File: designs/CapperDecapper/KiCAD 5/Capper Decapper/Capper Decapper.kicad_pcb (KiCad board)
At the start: 2 copper layers, 94 x 61.6 mm, 50 parts, among them J1 Screw_Terminal_01x02, J2 Conn_01x03_Female, J3 Analog_Zero, J4 Pi_Signals, J5 Motor_Power, Q1 Q_NMOS_GDS, U1 L2293, U10 INA214, U11 L2293, U12 INA214, U13 INA214, U14 LM338-ADJ, U2 INA214, U3 INA214, U4 L2293, U5 INA214, U6 INA214, U7 ADP172, U8 L2293, U9 INA214

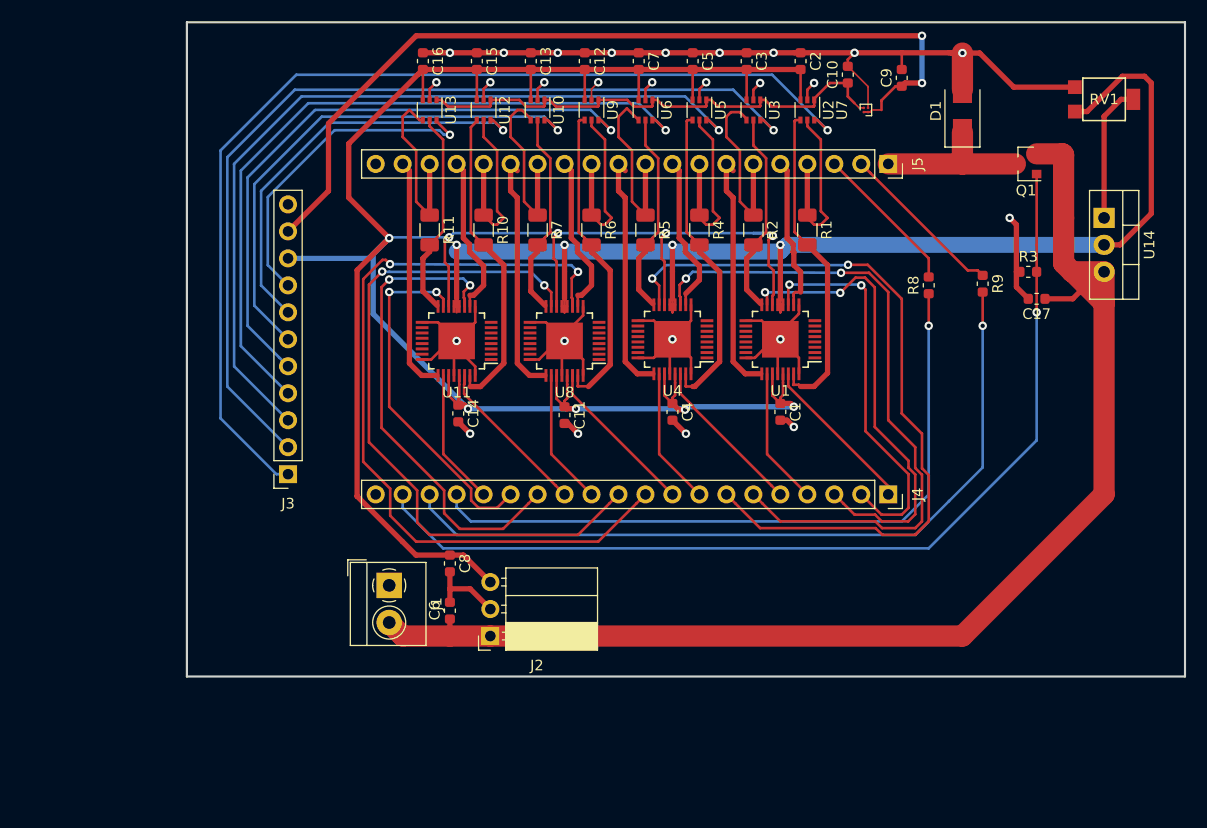
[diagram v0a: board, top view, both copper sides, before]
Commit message: PWM capper decapper board
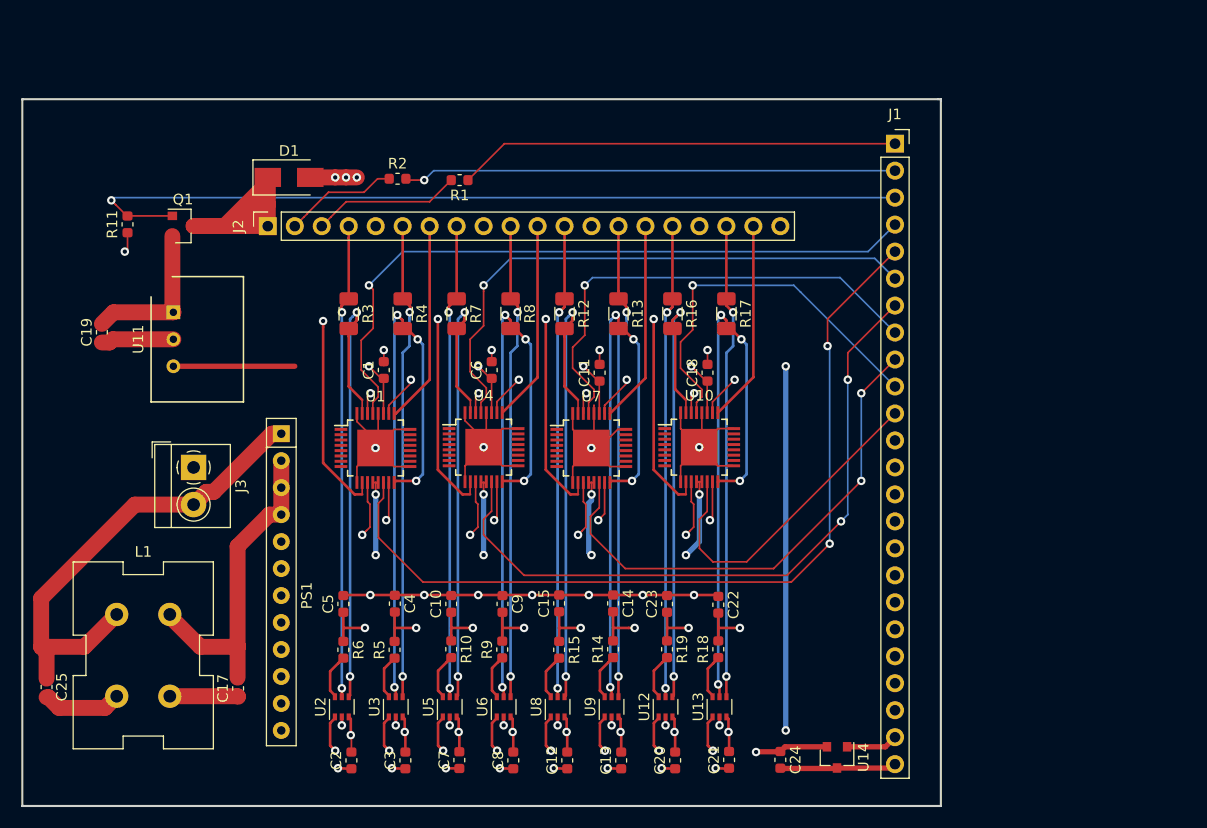
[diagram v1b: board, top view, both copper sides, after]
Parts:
- removed C16: C, Capacitor_SMD:C_0603_1608Metric
- removed J4: Pi_Signals, Connector_PinSocket_2.54mm:PinSocket_1x20_P2.54mm_Vertical
- removed J5: Motor_Power, Connector_PinSocket_2.54mm:PinSocket_1x20_P2.54mm_Vertical
- removed RV1: R_POT, CustomFootprints:R_TRIM_4mm_Gull
- added C18: 0.01uF, Capacitor_SMD:C_0603_1608Metric, F.Cu at (148.1, 60.3)
- added C19: 0.1uF, Capacitor_SMD:C_0603_1608Metric, F.Cu at (91.1, 56.5)
- added C20: 0.1uF, Capacitor_SMD:C_0603_1608Metric, F.Cu at (145.0, 96.8)
- added C21: 0.1uF, Capacitor_SMD:C_0603_1608Metric, F.Cu at (150.1, 96.7)
- added C22: 22nF, Capacitor_SMD:C_0603_1608Metric, F.Cu at (149.1, 82.1)
- added C23: 22nF, Capacitor_SMD:C_0603_1608Metric, F.Cu at (144.3, 82.1)
- added C24: 0.01uF, Capacitor_SMD:C_0603_1608Metric, F.Cu at (154.9, 96.7)
- added C25: 33uF, Capacitor_SMD:C_0603_1608Metric, F.Cu at (85.9, 89.9)
- added L1: L_Coupled, Inductor_THT:L_CommonMode_Wuerth_WE-CMB-S, F.Cu at (92.5, 83.1)
- added PS1: R-7XX, Resistor_THT:R_Array_SIP12, F.Cu at (108.0, 66.0)
- added R12: 0.05R, Resistor_SMD:R_1206_3216Metric, F.Cu at (134.6, 54.7)
- added R13: 0.05R, Resistor_SMD:R_1206_3216Metric, F.Cu at (139.7, 54.7)
- added R14: 20k, Resistor_SMD:R_0603_1608Metric, F.Cu at (139.2, 86.3)
- added R15: 20k, Resistor_SMD:R_0603_1608Metric, F.Cu at (134.1, 86.4)
- added R16: 0.05R, Resistor_SMD:R_1206_3216Metric, F.Cu at (144.8, 54.7)
- added R17: 0.05R, Resistor_SMD:R_1206_3216Metric, F.Cu at (149.9, 54.7)
- added R18: 20k, Resistor_SMD:R_0603_1608Metric, F.Cu at (149.1, 86.3)
- added R19: 20K, Resistor_SMD:R_0603_1608Metric, F.Cu at (144.3, 86.3)
- C1, C11, C7: value C -> 0.01uF
- C10, C14, C15, C4, C5, C9: value C -> 22nF
- C12, C13, C2, C3, C6, C8: value C -> 0.1uF
- C17: value C -> 33uF
- D1: value D_Schottky_Small_ALT -> Schottky
- J1: value Screw_Terminal_01x02 -> Pi Control Signals; footprint TerminalBlock_4Ucon:TerminalBlock_4Ucon_1x02_P3.50mm_Horizontal -> Connector_PinSocket_2.54mm:PinSocket_1x24_P2.54mm_Vertical
- J2: value Conn_01x03_Female -> Motor_Power; footprint Connector_PinSocket_2.54mm:PinSocket_1x03_P2.54mm_Horizontal -> Connector_PinSocket_2.54mm:PinSocket_1x20_P2.54mm_Vertical
- J3: value Analog_Zero -> Screw_Term; footprint Connector_PinSocket_2.54mm:PinSocket_1x11_P2.54mm_Vertical -> TerminalBlock_4Ucon:TerminalBlock_4Ucon_1x02_P3.50mm_Horizontal
- R1, R2: value R_US -> 330R; footprint Resistor_SMD:R_1206_3216Metric -> Resistor_SMD:R_0603_1608Metric
- R10, R5, R6: value R_US -> 20k; footprint Resistor_SMD:R_1206_3216Metric -> Resistor_SMD:R_0603_1608Metric
- R11: value R_US -> 5k; footprint Resistor_SMD:R_1206_3216Metric -> Resistor_SMD:R_0603_1608Metric
- R3, R8: value R_US -> 0.05R; footprint Resistor_SMD:R_0603_1608Metric -> Resistor_SMD:R_1206_3216Metric
- R4, R7: value R_US -> 0.05R
- R9: value R_US -> 20k
- U10: value INA214 -> L2293; footprint Package_TO_SOT_SMD:SOT-363_SC-70-6 -> Package_QFP:LQFP-32-1EP_5x5mm_P0.5mm_EP3.45x3.45mm
- U11: value L2293 -> V7805-1500R; footprint Package_QFP:LQFP-32-1EP_5x5mm_P0.5mm_EP3.45x3.45mm -> Package_SIP:SIP3_11.6x8.5mm
- U14: value LM338-ADJ -> MAX6018BEUR16; footprint Package_TO_SOT_THT:TO-220-3_Vertical -> Package_TO_SOT_SMD:SOT-23
- U7: value ADP172 -> L2293; footprint Package_BGA:WLP-4_0.86x0.86mm_P0.4mm -> Package_QFP:LQFP-32-1EP_5x5mm_P0.5mm_EP3.45x3.45mm
- U8: value L2293 -> INA214; footprint Package_QFP:LQFP-32-1EP_5x5mm_P0.5mm_EP3.45x3.45mm -> Package_TO_SOT_SMD:SOT-363_SC-70-6
- moved C17 83.7 mm to (103.9, 90.0), turned to 90 degrees
- moved Q1 79.6 mm to (98.7, 46.5), turned to 0 degrees
- moved C2 78.2 mm to (114.6, 96.8), turned to 90 degrees
- moved C3 73.3 mm to (119.6, 96.8), turned to 90 degrees
- moved U2 71.3 mm to (113.7, 91.8), turned to 90 degrees
- moved C7 67.9 mm to (124.7, 96.8), turned to 90 degrees
- moved C13 66.4 mm to (140.0, 96.8), turned to 90 degrees
- moved C12 65.9 mm to (134.9, 96.8), turned to 90 degrees
- moved U3 65.5 mm to (118.7, 91.8), turned to 90 degrees
- moved R3 64.1 mm to (114.3, 54.7), turned to 270 degrees
- moved D1 63.7 mm to (108.7, 41.9), turned to 0 degrees
- moved J1 63.2 mm to (165.7, 38.7), turned to 0 degrees
- moved U13 62.5 mm to (149.2, 91.8), turned to 90 degrees
- moved C10 62.3 mm to (124.0, 82.1)
- moved C9 62.2 mm to (128.8, 82.1), turned to 270 degrees
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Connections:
- C10 pad 1: /V_mon -> /ADC3
- C14 pad 1: /5V -> GND
- C14 pad 2: GND -> /ADC6
- C15 pad 1: GND -> /ADC5
- C15 pad 2: /5V -> GND
- C17 pad 1: +36V -> GND
- C17 pad 2: GND -> Net-(C17-Pad2)
- C4 pad 1: /5V -> GND
- C4 pad 2: GND -> /ADC2
- C5 pad 1: GND -> /ADC1
- C5 pad 2: /5V -> GND
- C6 pad 1: +36V -> /5V
- C8 pad 1: /5V -> GND
- C8 pad 2: GND -> /5V
- C9 pad 1: /3.3V -> GND
- C9 pad 2: GND -> /ADC4
- J1 pad 1: GND -> Net-(J1-Pad1)
- J1 pad 2: +36V -> Net-(J1-Pad2)
- J2 pad 1: +36V -> /SOL+
- J2 pad 2: GND -> /SW1
- J2 pad 3: /5V -> /SW2
- J3 pad 1: /ADC1 -> GND
- J3 pad 2: /ADC2 -> VBUS
- Q1 pad 2: +36V -> VBUS
- R1 pad 1: /MOT1_1 -> Net-(J1-Pad1)
- R1 pad 2: Net-(R1-Pad2) -> /SW2
- R10 pad 1: /MOT7_1 -> /ADC3
- R11 pad 1: /MOT8_1 -> GND
- R11 pad 2: Net-(R11-Pad2) -> /SOLSET
- R2 pad 1: /MOT2_1 -> /SW1
- R2 pad 2: Net-(R2-Pad2) -> Net-(J1-Pad2)
- R3 pad 1: GND -> /MOT1_1
- R3 pad 2: /SOLSET -> Net-(R3-Pad2)
- R4 pad 1: /MOT3_1 -> /MOT2_1
- R5 pad 1: /MOT4_1 -> Net-(R5-Pad1)
- R5 pad 2: Net-(R5-Pad2) -> /ADC2
- R6 pad 1: /MOT5_1 -> /ADC1
- R7 pad 1: /MOT6_1 -> /MOT3_1
- R8 pad 1: Net-(J4-Pad17) -> /MOT4_1
- R8 pad 2: /SW2 -> Net-(R8-Pad2)
- R9 pad 1: /SW1 -> Net-(R9-Pad1)
- R9 pad 2: Net-(J4-Pad18) -> /ADC4
- U1 pad 11: /MOT1_REV -> /REV
- U1 pad 14: /5V -> /EN2
- U1 pad 15: /MOT2_FWD -> /FWD
- U1 pad 16: Net-(R2-Pad2) -> Net-(R4-Pad2)
- U1 pad 26: /MOT2_REV -> /REV
- U1 pad 29: /5V -> /EN1
- U1 pad 30: /MOT1_FWD -> /FWD
- U1 pad 31: Net-(R1-Pad2) -> Net-(R3-Pad2)
- U10 pad 1: /V_mon -> Net-(U10-Pad1)
- U10 pad 2: GND -> Net-(U10-Pad2)
- U10 pad 3: /5V -> Net-(U10-Pad3)
- U10 pad 4: /MOT6_1 -> Net-(U10-Pad4)
- U10 pad 5: Net-(R7-Pad2) -> Net-(U10-Pad5)
- U10 pad 6: /ADC6 -> Net-(U10-Pad6)
- U11 pad 1: Net-(U11-Pad1) -> VBUS
- U11 pad 2: Net-(U11-Pad2) -> GND
- U11 pad 3: Net-(U11-Pad3) -> /5V
- U12 pad 4: Net-(R10-Pad2) -> Net-(R16-Pad2)
- U12 pad 6: /ADC7 -> Net-(R19-Pad2)
- U13 pad 5: Net-(R11-Pad2) -> Net-(R17-Pad2)
- U13 pad 6: /ADC8 -> Net-(R18-Pad1)
- U14 pad 1: Net-(RV1-Pad2) -> /3.3V
- U14 pad 2: /V_motor -> /V_mon
- U14 pad 3: +36V -> GND
- U2 pad 4: Net-(R1-Pad2) -> Net-(R3-Pad2)
- U2 pad 6: /ADC1 -> Net-(R6-Pad2)
- U3 pad 5: Net-(R2-Pad2) -> Net-(R4-Pad2)
- U3 pad 6: /ADC2 -> Net-(R5-Pad1)
- U4 pad 11: /MOT3_REV -> /REV
- U4 pad 14: /5V -> /EN4
- U4 pad 15: /MOT4_FWD -> /FWD
- U4 pad 16: Net-(R5-Pad2) -> Net-(R8-Pad2)
- U4 pad 26: /MOT4_REV -> /REV
- U4 pad 29: /5V -> /EN3
- U4 pad 30: /MOT3_FWD -> /FWD
- U4 pad 31: Net-(R4-Pad2) -> Net-(R7-Pad2)
- U5 pad 4: Net-(R4-Pad2) -> Net-(R7-Pad2)
- U5 pad 6: /ADC3 -> Net-(R10-Pad2)
- U6 pad 5: Net-(R5-Pad2) -> Net-(R8-Pad2)
- U6 pad 6: /ADC4 -> Net-(R9-Pad1)
- U8 pad 1: Net-(U8-Pad1) -> /V_mon
- U8 pad 2: Net-(U8-Pad2) -> GND
- U8 pad 3: Net-(U8-Pad3) -> /5V
- U8 pad 4: Net-(U8-Pad4) -> Net-(R12-Pad2)
- U8 pad 5: Net-(U8-Pad5) -> /MOT5_1
- U9 pad 4: Net-(R6-Pad2) -> /MOT6_1
- U9 pad 5: /MOT5_1 -> Net-(R13-Pad2)
- U9 pad 6: /ADC5 -> Net-(R14-Pad1)
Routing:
- net /REV: track 0.00 -> 143.7 mm, vias 0 -> 8
- net VBUS: track 0.00 -> 127.0 mm
- net /FWD: track 0.00 -> 125.4 mm, vias 0 -> 8
- net +36V: track 121.8 -> 0.00 mm
- net /EN2: track 0.00 -> 81.3 mm, vias 0 -> 2
- net /3.3V: track 82.6 -> 4.89 mm, vias 2 -> 0
- net /MOT5_REV: track 75.3 -> 0.00 mm, vias 2 -> 0
- net Net-(J4-Pad18): track 73.5 -> 0.00 mm, vias 1 -> 0
- net /5V: track 277.5 -> 205.2 mm, vias 9 -> 14
- net /MOT4_FWD: track 71.3 -> 0.00 mm, vias 2 -> 0
- net Net-(J4-Pad17): track 66.2 -> 0.00 mm, vias 1 -> 0
- net /EN1: track 0.00 -> 65.5 mm, vias 0 -> 1
- net /MOT6_FWD: track 65.1 -> 0.00 mm, vias 2 -> 0
- net /EN4: track 0.00 -> 65.1 mm, vias 0 -> 2
- net /MOT3_REV: track 63.3 -> 0.00 mm, vias 2 -> 0
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- added copper zone on In2.Cu, net GND
- removed copper zone on B.Cu, net GND
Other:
- board size 94 x 61.6 mm -> 86.5 x 66.5 mm
- copper layers 2 -> 4
- net class Default: clearance 0.18 -> 0.25
- rule trace_clearance: 0.18 -> 0.25
